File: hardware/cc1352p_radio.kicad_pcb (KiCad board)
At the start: 2 copper layers, 50.5 x 31 mm, 63 parts, among them J1 Conn_01x14_Female, J2 Conn_01x14_Female, J3 Conn_Coaxial, J4 Conn_02x05_Odd_Even, J5 USB_B_Micro, J6 Conn_01x02_Male, Q1 DMG2305UX-13, U1 CC1352PF3RGZ, U2 0900PC15A0036, U3 0900PC15A0036, U4 SKY13317-373, U5 TPS79601DR, Y1 48MHz, Y2 32.768kHz

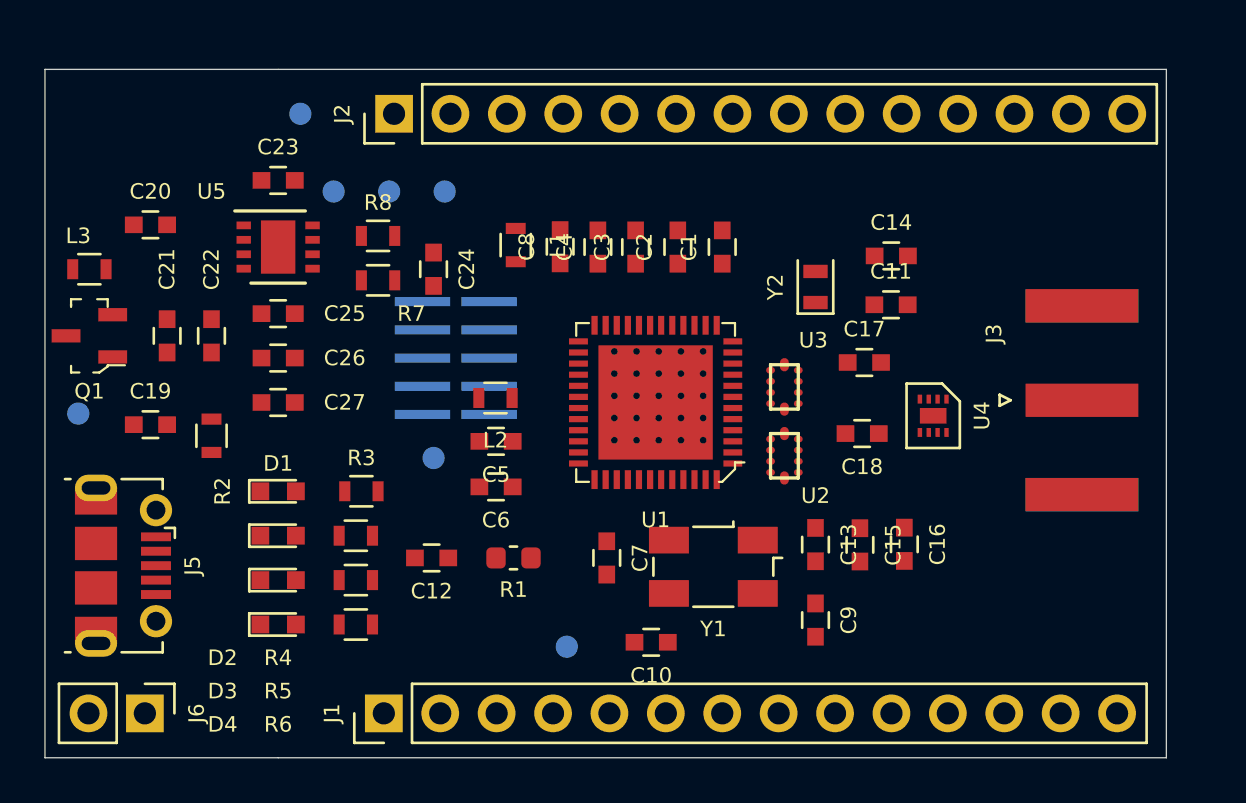
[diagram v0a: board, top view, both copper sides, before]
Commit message: Routed the board out. Might work.
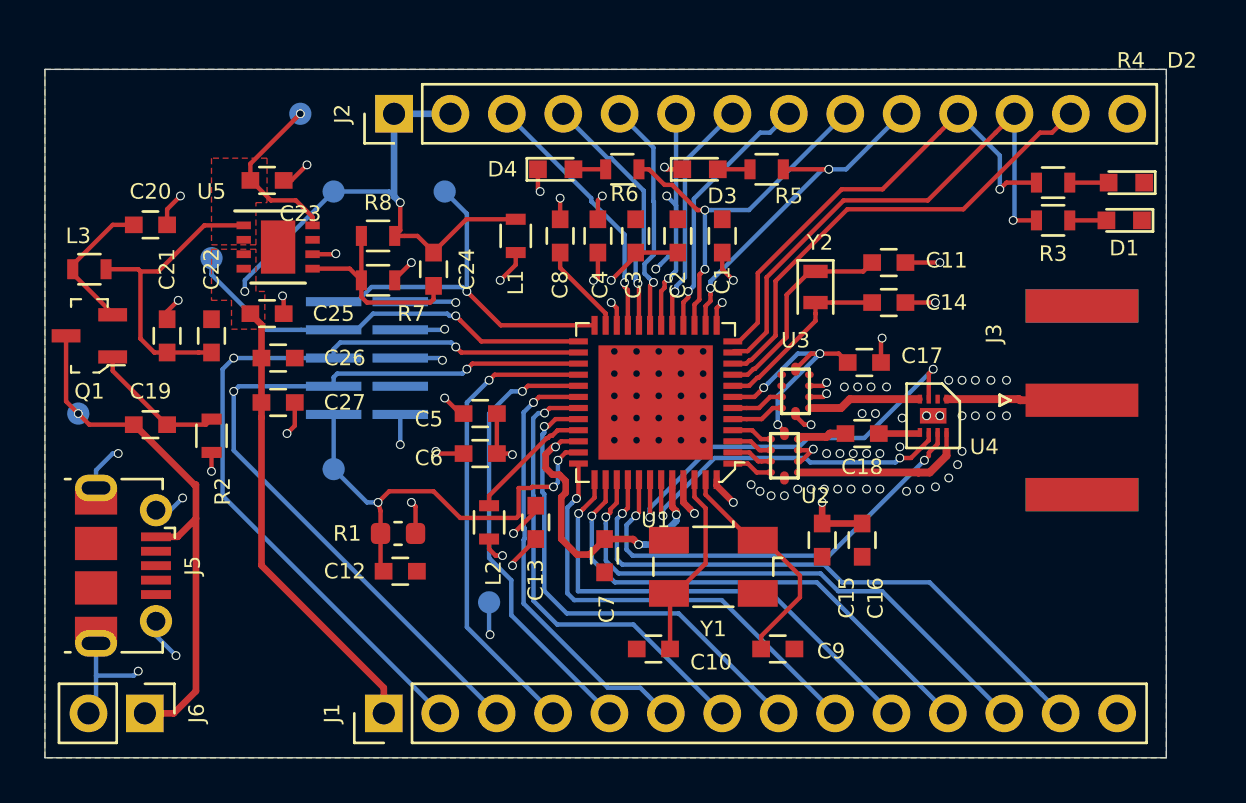
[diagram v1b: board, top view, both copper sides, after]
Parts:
- moved D2 41.4 mm to (208.2, 111.1), turned to 180 degrees
- moved D1 40.0 mm to (208.1, 112.8), turned to 180 degrees
- moved R4 35.2 mm to (204.9, 111.1), turned to 0 degrees
- moved R3 33.5 mm to (204.9, 112.8), turned to 0 degrees
- moved D3 26.5 mm to (189.0, 110.5)
- moved R5 26.2 mm to (192.0, 110.5)
- moved D4 24.0 mm to (182.5, 110.5)
- moved R6 23.8 mm to (185.5, 110.5)
- moved TP5 13.2 mm to (172.5, 124.0)
- moved C13 12.6 mm to (181.6, 126.4), turned to 90 degrees
- moved TP4 8.54 mm to (167.0, 114.5)
- moved TP7 6.96 mm to (179.5, 130.0)
- moved L2 5.61 mm to (179.5, 126.4), turned to 270 degrees
- moved R1 5.32 mm to (175.4, 126.9)
- moved J4 4.00 mm to (174.0, 119.0)
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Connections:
- J4 pad 1: VCC -> VDD
- U4 pad 9: (no net) -> GND
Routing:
- net VCC: track 0.00 -> 44.8 mm, vias 0 -> 2
- net GND: track 0.00 -> 41.7 mm, vias 0 -> 68
- net /DIO16: track 0.00 -> 36.5 mm, vias 0 -> 2
- net /DIO17: track 0.00 -> 35.7 mm, vias 0 -> 2
- net VDD: track 0.00 -> 31.2 mm, vias 0 -> 12
- net Net-(J1-Pad13): track 0.00 -> 26.6 mm, vias 0 -> 1
- net Net-(J1-Pad12): track 0.00 -> 24.6 mm, vias 0 -> 1
- net Net-(C19-Pad1): track 0.00 -> 24.5 mm, vias 0 -> 1
- net /DIO6: track 0.00 -> 24.5 mm, vias 0 -> 1
- net Net-(J1-Pad11): track 0.00 -> 22.8 mm, vias 0 -> 1
- net Net-(J1-Pad8): track 0.00 -> 22.0 mm, vias 0 -> 1
- net Net-(J1-Pad10): track 0.00 -> 21.7 mm, vias 0 -> 1
- net /DIO7: track 0.00 -> 21.7 mm, vias 0 -> 1
- net VBUS: track 0.00 -> 21.4 mm, vias 0 -> 1
- net Net-(J2-Pad13): track 0.00 -> 21.3 mm
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- added copper zone on B.Cu, net GND
- added copper zone on F.Cu, net GND
- added copper zone on In1.Cu, net GND
- added copper zone on F.Cu, net VBUS
- added copper zone on F.Cu, net VCC
- added copper zone on In2.Cu, net VDD
- added copper zone on In2.Cu, net VDDF
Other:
- copper layers 2 -> 4
- net class Default: via_dia 0.8 -> 0.4; via_drill 0.4 -> 0.3
- rule via_min_drill: 0.3 -> 0.1
- rule via_min_size: 0.4 -> 0.2
- board text added: "RAW_PWR"
- board text added: "RESET_N"
- board text added: "TCKC"
- board text added: "TMSC"
- board text added: "VBUS"
- board text added: "VCC"
- board text added: "VDDF"
